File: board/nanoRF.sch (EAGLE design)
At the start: 19 parts

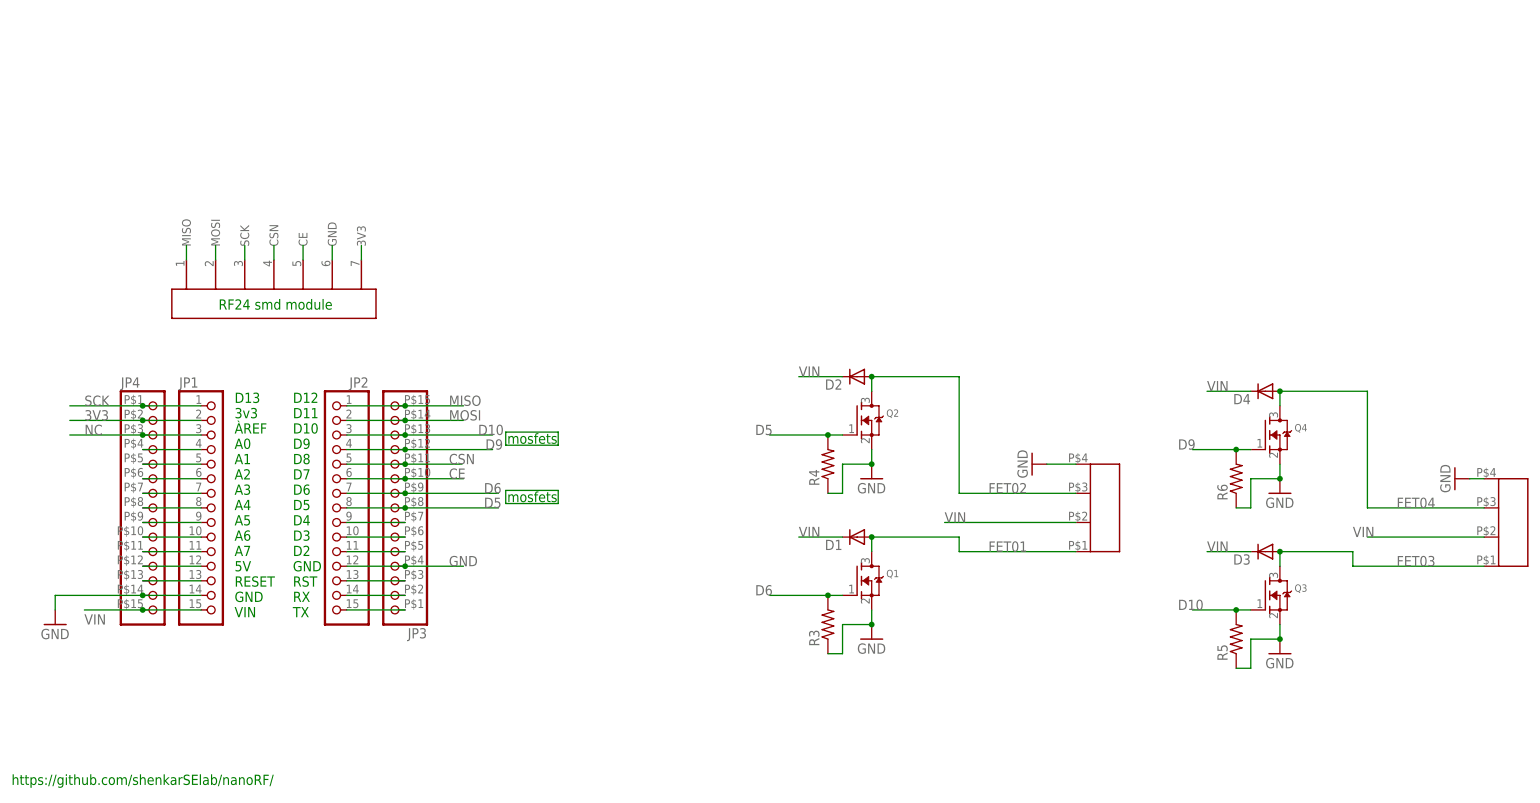
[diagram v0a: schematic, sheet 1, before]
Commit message: added schema
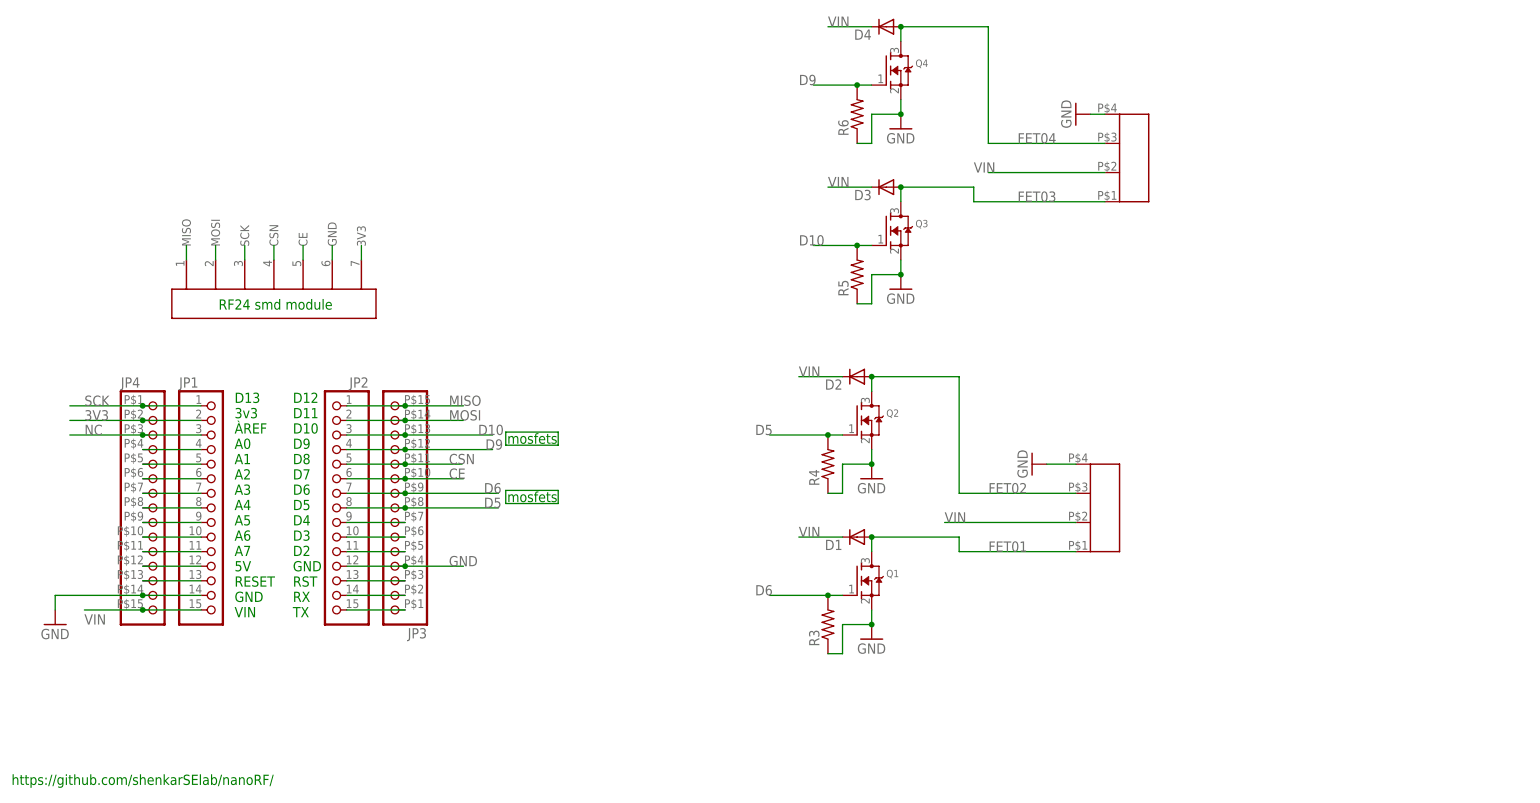
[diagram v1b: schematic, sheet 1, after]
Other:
- moved on the sheet: D3, D4, Q3, Q4, R5, R6
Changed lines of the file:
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@@
 <part name="JP3" library="nano24rf" deviceset="HEADER-1X15" device="LONG"/>
 <part name="JP4" library="nano24rf" deviceset="HEADER-1X15" device="LONG"/>
+<part name="FRAME1" library="frames" library_urn="urn:adsk.eagle:library:229" deviceset="A4L-LOC" device=""/>
 </parts>
 <sheets>
@@
 <instance part="D2" gate="D" x="157.48" y="71.12" rot="R180"/>
 <instance part="U$1" gate="1" x="160.02" y="53.34"/>
-<instance part="Q3" gate="G$1" x="228.6" y="33.02"/>
-<instance part="D3" gate="D" x="228.6" y="40.64" smashed="yes" rot="R180">
-<attribute name="NAME" x="226.06" y="40.1574" size="1.778" layer="95" rot="R180"/>
-<attribute name="VALUE" x="226.06" y="42.9514" size="1.778" layer="96" rot="R180"/>
+<instance part="Q3" gate="G$1" x="162.56" y="96.52"/>
+<instance part="D3" gate="D" x="162.56" y="104.14" smashed="yes" rot="R180">
+<attribute name="NAME" x="160.02" y="103.6574" size="1.778" layer="95" rot="R180"/>
+<attribute name="VALUE" x="160.02" y="106.4514" size="1.778" layer="96" rot="R180"/>
 </instance>
-<instance part="U$2" gate="1" x="231.14" y="22.86"/>
-<instance part="Q4" gate="G$1" x="228.6" y="60.96"/>
-<instance part="D4" gate="D" x="228.6" y="68.58" rot="R180"/>
-<instance part="U$4" gate="1" x="231.14" y="50.8"/>
-<instance part="MOSFET-34" gate="G$1" x="269.24" y="43.18" rot="R90"/>
+<instance part="U$2" gate="1" x="165.1" y="86.36"/>
+<instance part="Q4" gate="G$1" x="162.56" y="124.46"/>
+<instance part="D4" gate="D" x="162.56" y="132.08" rot="R180"/>
+<instance part="U$4" gate="1" x="165.1" y="114.3"/>
+<instance part="MOSFET-34" gate="G$1" x="203.2" y="106.68" rot="R90"/>
 <instance part="MOSFET-12" gate="G$1" x="198.12" y="45.72" rot="R90"/>
 <instance part="R4" gate="G$1" x="152.4" y="55.88" rot="R90"/>
 <instance part="R3" gate="G$1" x="152.4" y="27.94" rot="R90"/>
-<instance part="R6" gate="G$1" x="223.52" y="53.34" rot="R90"/>
-<instance part="R5" gate="G$1" x="223.52" y="25.4" rot="R90"/>
-<instance part="U$9" gate="1" x="261.62" y="53.34" rot="R270"/>
+<instance part="R6" gate="G$1" x="157.48" y="116.84" rot="R90"/>
+<instance part="R5" gate="G$1" x="157.48" y="88.9" rot="R90"/>
+<instance part="U$9" gate="1" x="195.58" y="116.84" rot="R270"/>
 <instance part="U$10" gate="1" x="187.96" y="55.88" rot="R270"/>
 <instance part="JP3" gate="G$1" x="76.2" y="48.26" rot="R180"/>
 <instance part="JP4" gate="G$1" x="35.56" y="48.26"/>
+<instance part="FRAME1" gate="G$1" x="2.54" y="-17.78"/>
 </instances>
 <busses>
@@
 <pinref part="Q3" gate="G$1" pin="S"/>
 <pinref part="U$2" gate="1" pin="GND"/>
-<wire x1="231.14" y1="25.4" x2="231.14" y2="27.94" width="0.1524" layer="91"/>
+<wire x1="165.1" y1="88.9" x2="165.1" y2="91.44" width="0.1524" layer="91"/>
 <pinref part="R5" gate="G$1" pin="1"/>
-<wire x1="223.52" y1="20.32" x2="226.06" y2="20.32" width="0.1524" layer="91"/>
-<wire x1="226.06" y1="20.32" x2="226.06" y2="25.4" width="0.1524" layer="91"/>
-<wire x1="226.06" y1="25.4" x2="231.14" y2="25.4" width="0.1524" layer="91"/>
-<junction x="231.14" y="25.4"/>
+<wire x1="157.48" y1="83.82" x2="160.02" y2="83.82" width="0.1524" layer="91"/>
+<wire x1="160.02" y1="83.82" x2="160.02" y2="88.9" width="0.1524" layer="91"/>
+<wire x1="160.02" y1="88.9" x2="165.1" y2="88.9" width="0.1524" layer="91"/>
+<junction x="165.1" y="88.9"/>
 </segment>
 <segment>
 <pinref part="Q4" gate="G$1" pin="S"/>
 <pinref part="U$4" gate="1" pin="GND"/>
-<wire x1="231.14" y1="53.34" x2="231.14" y2="55.88" width="0.1524" layer="91"/>
+<wire x1="165.1" y1="116.84" x2="165.1" y2="119.38" width="0.1524" layer="91"/>
 <pinref part="R6" gate="G$1" pin="1"/>
-<wire x1="223.52" y1="48.26" x2="226.06" y2="48.26" width="0.1524" layer="91"/>
-<wire x1="226.06" y1="48.26" x2="226.06" y2="53.34" width="0.1524" layer="91"/>
-<wire x1="226.06" y1="53.34" x2="231.14" y2="53.34" width="0.1524" layer="91"/>
-<junction x="231.14" y="53.34"/>
+<wire x1="157.48" y1="111.76" x2="160.02" y2="111.76" width="0.1524" layer="91"/>
+<wire x1="160.02" y1="111.76" x2="160.02" y2="116.84" width="0.1524" layer="91"/>
+<wire x1="160.02" y1="116.84" x2="165.1" y2="116.84" width="0.1524" layer="91"/>
+<junction x="165.1" y="116.84"/>
 </segment>
 <segment>
@@
 <pinref part="U$9" gate="1" pin="GND"/>
 <pinref part="MOSFET-34" gate="G$1" pin="P$4"/>
-<wire x1="264.16" y1="53.34" x2="266.7" y2="53.34" width="0.1524" layer="91"/>
+<wire x1="198.12" y1="116.84" x2="200.66" y2="116.84" width="0.1524" layer="91"/>
 </segment>
 </net>
@@
 </segment>
 <segment>
-<wire x1="266.7" y1="43.18" x2="246.38" y2="43.18" width="0.1524" layer="91"/>
-<label x="243.84" y="43.18" size="1.778" layer="95"/>
+<wire x1="200.66" y1="106.68" x2="180.34" y2="106.68" width="0.1524" layer="91"/>
+<label x="177.8" y="106.68" size="1.778" layer="95"/>
 <pinref part="MOSFET-34" gate="G$1" pin="P$2"/>
 </segment>
 <segment>
 <pinref part="D4" gate="D" pin="C"/>
-<wire x1="218.44" y1="68.58" x2="226.06" y2="68.58" width="0.1524" layer="91"/>
-<label x="218.44" y="68.58" size="1.778" layer="95"/>
+<wire x1="152.4" y1="132.08" x2="160.02" y2="132.08" width="0.1524" layer="91"/>
+<label x="152.4" y="132.08" size="1.778" layer="95"/>
 </segment>
 <segment>
 <pinref part="D3" gate="D" pin="C"/>
-<wire x1="226.06" y1="40.64" x2="218.44" y2="40.64" width="0.1524" layer="91"/>
-<label x="218.44" y="40.64" size="1.778" layer="95"/>
+<wire x1="160.02" y1="104.14" x2="152.4" y2="104.14" width="0.1524" layer="91"/>
+<label x="152.4" y="104.14" size="1.778" layer="95"/>
 </segment>
 </net>
@@
 </segment>
 <segment>
-<label x="213.36" y="58.42" size="1.778" layer="95"/>
+<label x="147.32" y="121.92" size="1.778" layer="95"/>
 <pinref part="Q4" gate="G$1" pin="G"/>
-<wire x1="223.52" y1="58.42" x2="226.06" y2="58.42" width="0.1524" layer="91"/>
+<wire x1="157.48" y1="121.92" x2="160.02" y2="121.92" width="0.1524" layer="91"/>
 <pinref part="R6" gate="G$1" pin="2"/>
-<wire x1="223.52" y1="58.42" x2="215.9" y2="58.42" width="0.1524" layer="91"/>
-<junction x="223.52" y="58.42"/>
+<wire x1="157.48" y1="121.92" x2="149.86" y2="121.92" width="0.1524" layer="91"/>
+<junction x="157.48" y="121.92"/>
 </segment>
 </net>
@@
 <pinref part="Q3" gate="G$1" pin="D"/>
 <pinref part="D3" gate="D" pin="A"/>
-<wire x1="231.14" y1="38.1" x2="231.14" y2="40.64" width="0.1524" layer="91"/>
-<junction x="231.14" y="40.64"/>
-<wire x1="266.7" y1="38.1" x2="243.84" y2="38.1" width="0.1524" layer="91"/>
-<wire x1="243.84" y1="38.1" x2="243.84" y2="40.64" width="0.1524" layer="91"/>
-<wire x1="243.84" y1="40.64" x2="231.14" y2="40.64" width="0.1524" layer="91"/>
+<wire x1="165.1" y1="101.6" x2="165.1" y2="104.14" width="0.1524" layer="91"/>
+<junction x="165.1" y="104.14"/>
+<wire x1="200.66" y1="101.6" x2="177.8" y2="101.6" width="0.1524" layer="91"/>
+<wire x1="177.8" y1="101.6" x2="177.8" y2="104.14" width="0.1524" layer="91"/>
+<wire x1="177.8" y1="104.14" x2="165.1" y2="104.14" width="0.1524" layer="91"/>
 <pinref part="MOSFET-34" gate="G$1" pin="P$1"/>
-<label x="251.46" y="38.1" size="1.778" layer="95"/>
+<label x="185.42" y="101.6" size="1.778" layer="95"/>
 </segment>
 </net>
@@
 <pinref part="Q4" gate="G$1" pin="D"/>
 <pinref part="D4" gate="D" pin="A"/>
-<wire x1="231.14" y1="66.04" x2="231.14" y2="68.58" width="0.1524" layer="91"/>
-<junction x="231.14" y="68.58"/>
-<wire x1="246.38" y1="68.58" x2="231.14" y2="68.58" width="0.1524" layer="91"/>
-<wire x1="266.7" y1="48.26" x2="246.38" y2="48.26" width="0.1524" layer="91"/>
-<wire x1="246.38" y1="48.26" x2="246.38" y2="68.58" width="0.1524" layer="91"/>
+<wire x1="165.1" y1="129.54" x2="165.1" y2="132.08" width="0.1524" layer="91"/>
+<junction x="165.1" y="132.08"/>
+<wire x1="180.34" y1="132.08" x2="165.1" y2="132.08" width="0.1524" layer="91"/>
+<wire x1="200.66" y1="111.76" x2="180.34" y2="111.76" width="0.1524" layer="91"/>
+<wire x1="180.34" y1="111.76" x2="180.34" y2="132.08" width="0.1524" layer="91"/>
 <pinref part="MOSFET-34" gate="G$1" pin="P$3"/>
-<label x="251.46" y="48.26" size="1.778" layer="95"/>
+<label x="185.42" y="111.76" size="1.778" layer="95"/>
 </segment>
 </net>
@@
 </segment>
 <segment>
-<label x="213.36" y="30.48" size="1.778" layer="95"/>
+<label x="147.32" y="93.98" size="1.778" layer="95"/>
 <pinref part="Q3" gate="G$1" pin="G"/>
-<wire x1="223.52" y1="30.48" x2="226.06" y2="30.48" width="0.1524" layer="91"/>
+<wire x1="157.48" y1="93.98" x2="160.02" y2="93.98" width="0.1524" layer="91"/>
 <pinref part="R5" gate="G$1" pin="2"/>
-<wire x1="215.9" y1="30.48" x2="223.52" y2="30.48" width="0.1524" layer="91"/>
-<junction x="223.52" y="30.48"/>
+<wire x1="149.86" y1="93.98" x2="157.48" y2="93.98" width="0.1524" layer="91"/>
+<junction x="157.48" y="93.98"/>
 </segment>
 </net>
@@
 which will not be processed correctly with this version.
 </note>
+<note version="8.2" severity="warning">
+Since Version 8.2, EAGLE supports online libraries. The ids
+of those online libraries will not be understood (or retained)
+with this version.
+</note>
+<note version="8.3" severity="warning">
+Since Version 8.3, EAGLE supports URNs for individual library
+assets (packages, symbols, and devices). The URNs of those assets
+will not be understood (or retained) with this version.
+</note>
 </compatibility>
